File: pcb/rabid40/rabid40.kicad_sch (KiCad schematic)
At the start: 30 parts

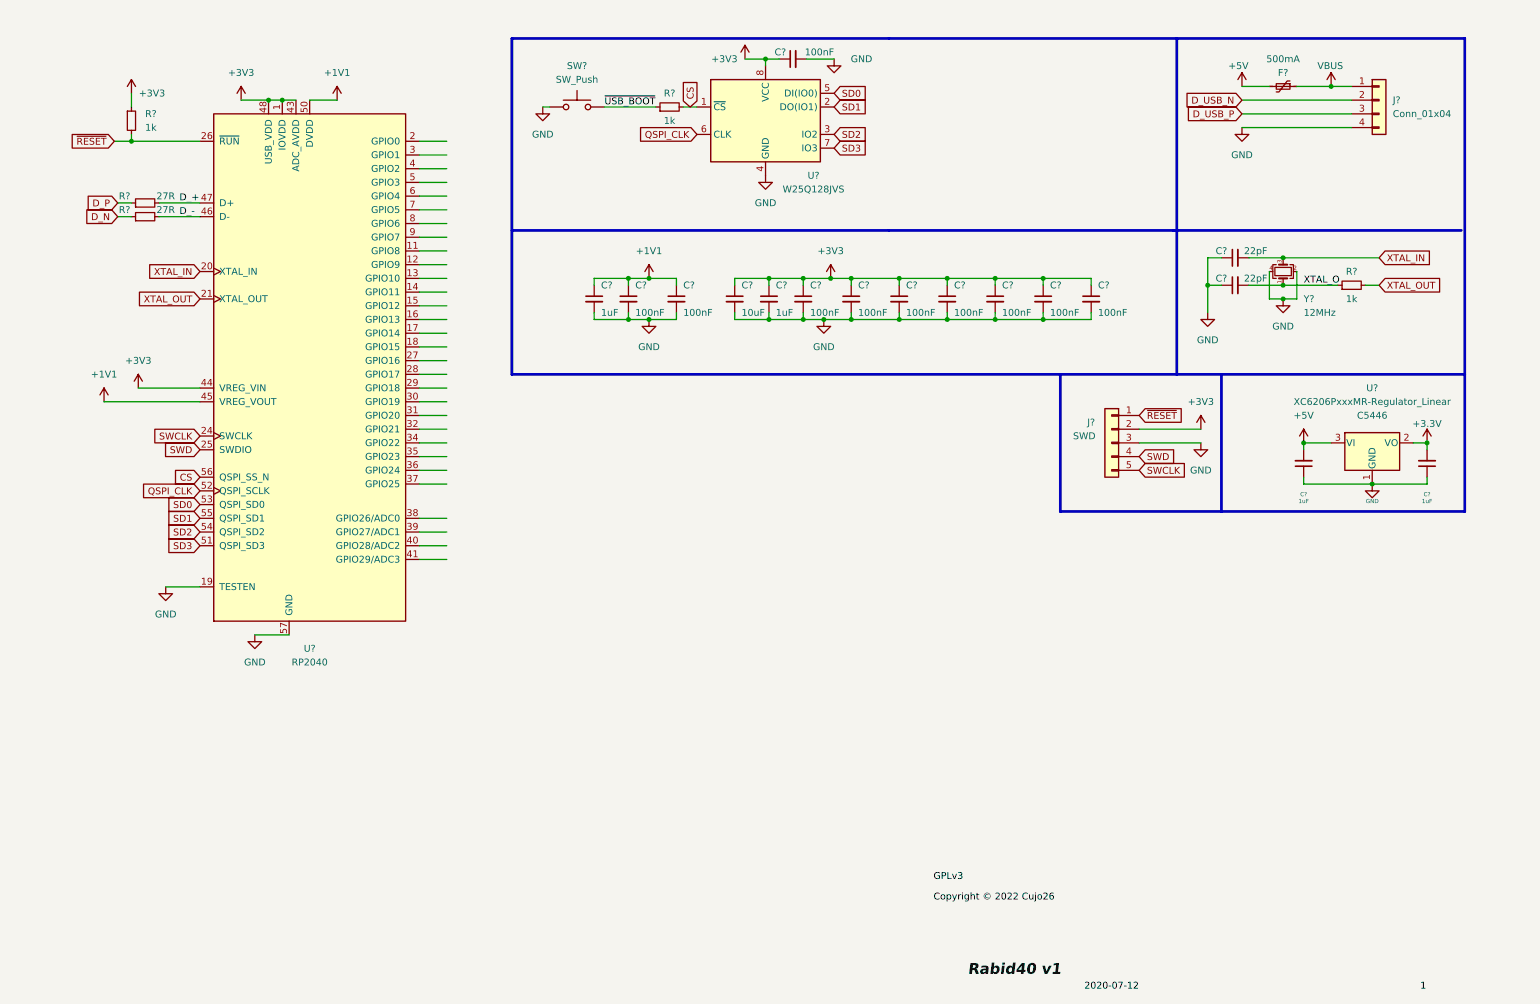
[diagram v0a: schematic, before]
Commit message: files organised
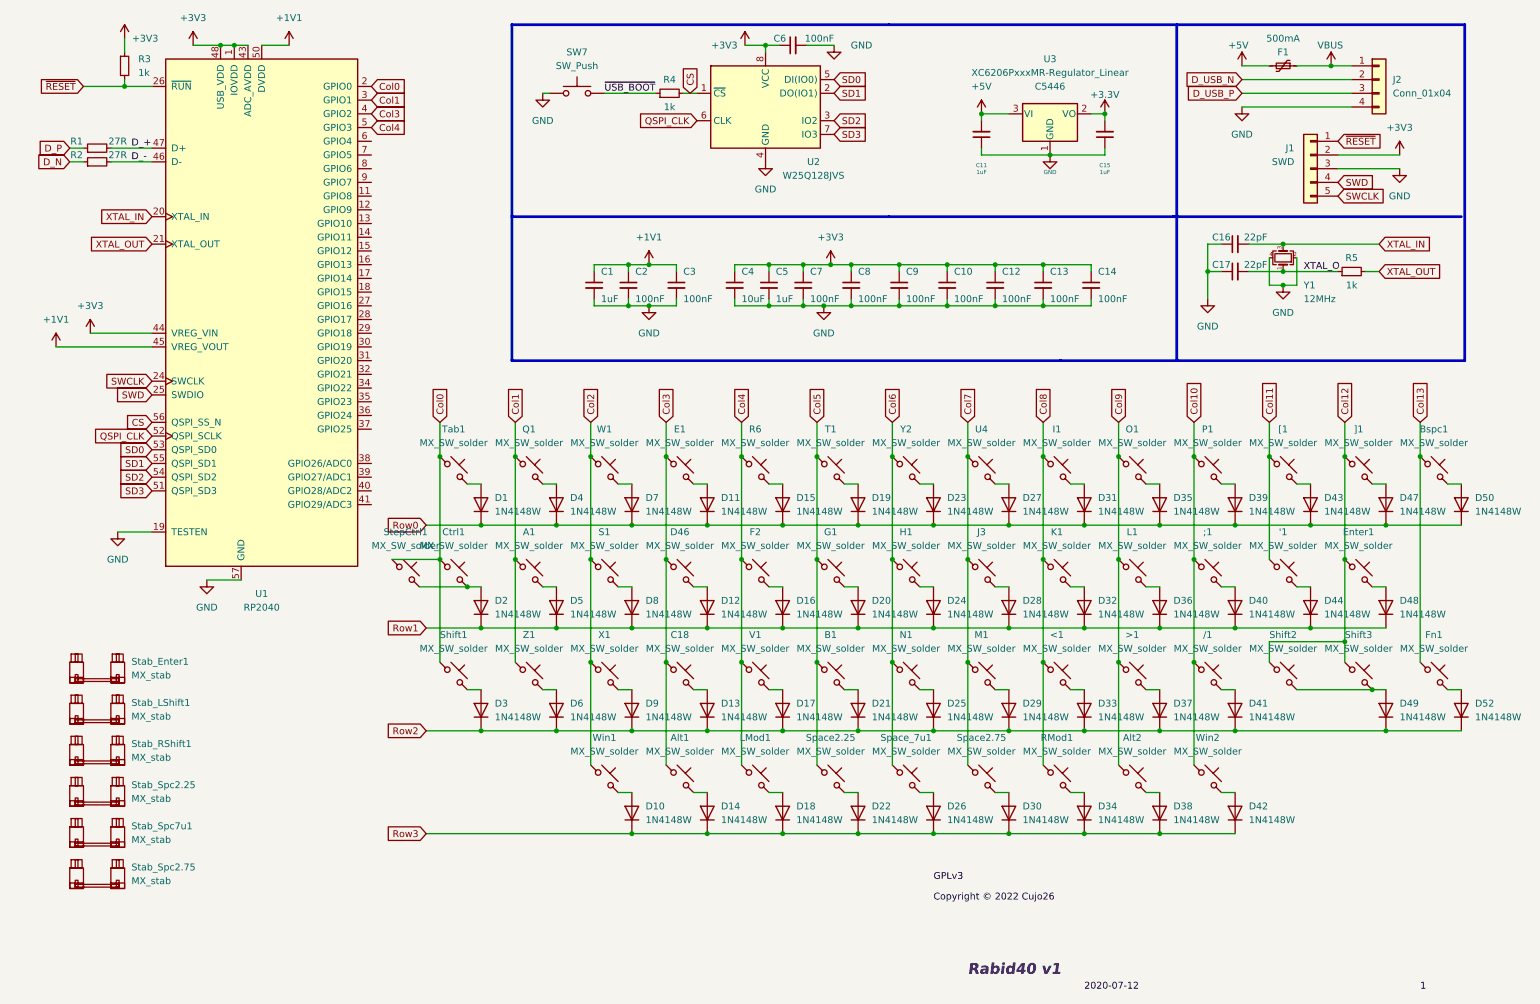
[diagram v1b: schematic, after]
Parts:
- removed C? (x2): 1uF, Capacitor_SMD:C_0402_1005Metric, symbol Device:C_Small
- removed J?: SWD, Connector_PinSocket_2.54mm:PinSocket_1x05_P2.54mm_Vertical, symbol Connector_Generic:Conn_01x05
- removed U?: XC6206PxxxMR-Regulator_Linear, Package_TO_SOT_SMD:SOT-23, symbol kicad-keyboard-parts:XC6206PxxxMR-Regulator_Linear
- added '1, /1, ;1, <1, >1, A1, Alt1, Alt2, B1, C18, D46, E1, Enter1, F2, Fn1, G1, H1, I1, J3, K1, L1, LMod1, M1, N1, O1, P1, Q1, R6, RMod1, S1, Shift1, Shift2, Shift3, Space2.25, Space2.75, Space_7u1, T1, U4, V1, W1, Win1, Win2, X1, Y2, Z1, [1, ]1: MX_SW_solder, marbastlib-mx:SW_MX_1u, symbol marbastlib-mx:MX_SW_solder
- added Bspc1, Tab1: MX_SW_solder, marbastlib-mx:SW_MX_1.5u, symbol marbastlib-mx:MX_SW_solder
- added C11, C15: 1uF, Capacitor_SMD:C_0402_1005Metric, symbol Device:C_Small
- added Ctrl1: MX_SW_solder, marbastlib-mx:SW_MX_1.75u, symbol marbastlib-mx:MX_SW_solder
- added D1, D10, D11, D12, D13, D14, D15, D16, D17, D18, D19, D2, D20, D21, D22, D23, D24, D25, D26, D27, D28, D29, D3, D30, D31, D32, D33, D34, D35, D36, D37, D38, D39, D4, D40, D41, D42, D43, D44, D47, D48, D49, D5, D50, D52, D6, D7, D8, D9: 1N4148W, Diode_SMD:D_SOD-123, symbol Diode:1N4148W
- added J1: SWD, Connector_PinSocket_2.54mm:PinSocket_1x05_P2.54mm_Vertical, symbol Connector_Generic:Conn_01x05
- added Stab_Enter1, Stab_LShift1: MX_stab, marbastlib-mx:STAB_MX_2.25u, symbol marbastlib-mx:MX_stab
- added Stab_RShift1: MX_stab, marbastlib-mx:STAB_MX_2.75u, symbol marbastlib-mx:MX_stab
- added Stab_Spc2.25: MX_stab, marbastlib-mx:STAB_MX_P_2.25u, symbol marbastlib-mx:MX_stab
- added Stab_Spc2.75: MX_stab, marbastlib-mx:STAB_MX_P_2.75u, symbol marbastlib-mx:MX_stab
- added Stab_Spc7u1: MX_stab, marbastlib-mx:STAB_MX_P_7u, symbol marbastlib-mx:MX_stab
- added StepCtrl1: MX_SW_solder, marbastlib-mx:SW_MX_1.75u_stp, symbol marbastlib-mx:MX_SW_solder
- added U3: XC6206PxxxMR-Regulator_Linear, Package_TO_SOT_SMD:SOT-23, symbol kicad-keyboard-parts:XC6206PxxxMR-Regulator_Linear
- J2: renamed from J?; footprint (none) -> Connector_JST:JST_EH_S4B-EH_1x04_P2.50mm_Horizontal
- U1: renamed from U?; footprint Sleep-Lib:RP2040-QFN-56 -> Sleep-lib:RP2040-QFN-56
- gave numbers to parts that had none: 24
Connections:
- net +3V3: now also C15.2, J1.2 (Pin_2), U3.2 (VO)
- net +5V: now also C11.2, U3.3 (VI)
- net GND: now also C11.1, C15.1, J1.3 (Pin_3), U3.1 (GND)
- net SWCLK: now also J1.5 (Pin_5)
- net SWD: now also J1.4 (Pin_4)
- net ~{RESET}: now also J1.1 (Pin_1)
- net Col0: now reaches U1.2 (GPIO0)
- net Col0: now also Ctrl1.1, Shift1.1, StepCtrl1.1, Tab1.1
- net Col1: now reaches U1.3 (GPIO1)
- net Col1: now also A1.1, Q1.1, Z1.1
- net Col3: now reaches U1.4 (GPIO2)
- net Col3: now also Alt1.1, C18.1, D46.1, E1.1
- net Col4: now reaches U1.5 (GPIO3)
- net Col4: now also F2.1, LMod1.1, R6.1, V1.1
- new net: A1.2, D5.2 (A)
- new net: D34.2 (A), RMod1.2
- new net: '1.2, D44.2 (A)
- new net: D48.2 (A), Enter1.2
- new net: D7.2 (A), W1.2
- new net: D31.2 (A), I1.2
- new net: B1.2, D21.2 (A)
- new net: D52.2 (A), Fn1.2
- new net: D15.2 (A), R6.2
- new net: D17.2 (A), V1.2
- new net: D8.2 (A), S1.2
- new net: D49.2 (A), Shift2.2, Shift3.2
- new net: D12.2 (A), D46.2
- new net: D39.2 (A), P1.2
- new net: D27.2 (A), U4.2
- new net: Ctrl1.2, D2.2 (A), StepCtrl1.2
- new net: D22.2 (A), Space2.25.2
- new net: D42.2 (A), Win2.2
- new net: D4.2 (A), Q1.2
- new net: >1.2, D37.2 (A)
- new net: D29.2 (A), M1.2
- new net: D6.2 (A), Z1.2
- new net: Alt1.2, D14.2 (A)
- new net: D47.2 (A), ]1.2
- new net: <1.2, D33.2 (A)
- new net: D1.2 (A), Tab1.2
- new net: D19.2 (A), T1.2
- new net: D36.2 (A), L1.2
- new net: D11.2 (A), E1.2
- new net: D10.2 (A), Win1.2
- new net: D28.2 (A), J3.2
- new net: D23.2 (A), Y2.2
- new net: Bspc1.2, D50.2 (A)
- new net: D16.2 (A), F2.2
- new net: D26.2 (A), Space_7u1.2
- new net: D35.2 (A), O1.2
- new net: Alt2.2, D38.2 (A)
- new net: /1.2, D41.2 (A)
- new net: D30.2 (A), Space2.75.2
- new net: D25.2 (A), N1.2
- new net: D3.2 (A), Shift1.2
- new net: D32.2 (A), K1.2
- new net: D43.2 (A), [1.2
- new net: D18.2 (A), LMod1.2
- new net: ;1.2, D40.2 (A)
- new net: D9.2 (A), X1.2
- new net: D20.2 (A), G1.2
- new net: C18.2, D13.2 (A)
- new net: D24.2 (A), H1.2
- new net Col10: /1.1, ;1.1, P1.1, Win2.1
- new net Col11: '1.1, [1.1
- new net Col12: Enter1.1, Shift2.1, Shift3.1, ]1.1
- new net Col13: Bspc1.1, Fn1.1
- new net Col2: S1.1, W1.1, Win1.1, X1.1
- new net Col5: B1.1, G1.1, Space2.25.1, T1.1
- new net Col6: H1.1, N1.1, Space_7u1.1, Y2.1
- new net Col7: J3.1, M1.1, Space2.75.1, U4.1
- new net Col8: <1.1, I1.1, K1.1, RMod1.1
- new net Col9: >1.1, Alt2.1, L1.1, O1.1
- new net Row0: D1.1 (K), D11.1 (K), D15.1 (K), D19.1 (K), D23.1 (K), D27.1 (K), D31.1 (K), D35.1 (K), D39.1 (K), D4.1 (K), D43.1 (K), D47.1 (K), D50.1 (K), D7.1 (K)
- new net Row1: D12.1 (K), D16.1 (K), D2.1 (K), D20.1 (K), D24.1 (K), D28.1 (K), D32.1 (K), D36.1 (K), D40.1 (K), D44.1 (K), D48.1 (K), D5.1 (K), D8.1 (K)
- new net Row2: D13.1 (K), D17.1 (K), D21.1 (K), D25.1 (K), D29.1 (K), D3.1 (K), D33.1 (K), D37.1 (K), D41.1 (K), D49.1 (K), D52.1 (K), D6.1 (K), D9.1 (K)
- new net Row3: D10.1 (K), D14.1 (K), D18.1 (K), D22.1 (K), D26.1 (K), D30.1 (K), D34.1 (K), D38.1 (K), D42.1 (K)
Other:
- moved on the sheet: C1, C10, C12, C13, C14, C16, C17, C2, C3, C4, C5, C6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
